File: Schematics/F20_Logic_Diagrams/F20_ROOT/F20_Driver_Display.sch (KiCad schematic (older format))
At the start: 2 parts, among them U5 StepDownConverter, U6 Driver_Display

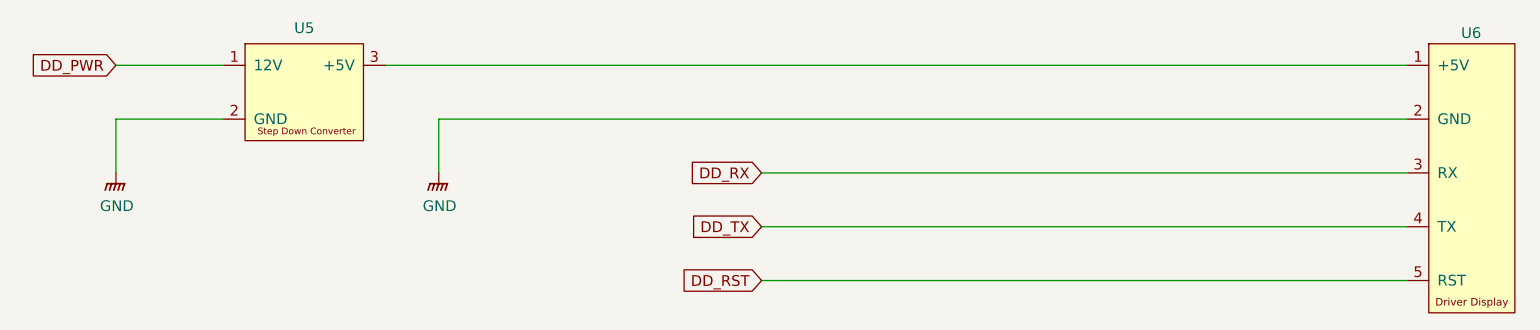
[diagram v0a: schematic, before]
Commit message: 02/18/20 update
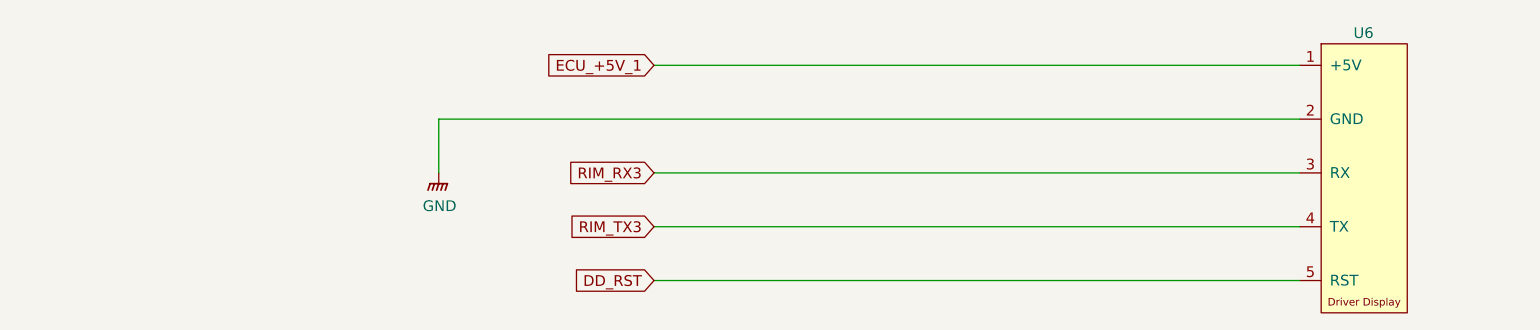
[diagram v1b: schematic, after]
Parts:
- removed U5: StepDownConverter, symbol FSAE_Library:StepDownConverter
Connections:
- net ECU_+5V_1: now reaches U6.1 (+5V)
- net DD_RX renamed RIM_RX3
- net DD_TX renamed RIM_TX3
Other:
- moved on the sheet: U6
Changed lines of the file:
@@
 $Descr A 11000 8500
 encoding utf-8
-Sheet 5 11
+Sheet 7 13
 Title "FSAE"
 Date "2020-02-03"
@@
 L FSAE_Library:Driver_Display U6
 U 1 1 5E291EA2
-P 8000 3000
-F 0 "U6" H 8250 3150 50  0000 L CNN
-F 1 "Driver_Display" H 8300 3150 50  0001 C CNN
-F 2 "" H 8300 3150 50  0001 C CNN
-F 3 "" H 8300 3150 50  0001 C CNN
-	1    8000 3000
-	1    0    0    -1
-$EndComp
-$Comp
-L FSAE_Library:StepDownConverter U5
-U 1 1 5E297DA5
-P 2500 3000
-F 0 "U5" H 2875 3173 50  0000 C CNN
-F 1 "StepDownConverter" H 2750 3150 50  0001 C CNN
-F 2 "" H 3000 3500 50  0001 C CNN
-F 3 "" H 3000 3500 50  0001 C CNN
-	1    2500 3000
+P 7500 3000
+F 0 "U6" H 7750 3150 50  0000 L CNN
+F 1 "Driver_Display" H 7800 3150 50  0001 C CNN
+F 2 "" H 7800 3150 50  0001 C CNN
+F 3 "" H 7800 3150 50  0001 C CNN
+	1    7500 3000
 	1    0    0    -1
 $EndComp
 Wire Wire Line
-	5000 3500 8000 3500
+	4500 3500 7500 3500
 Wire Wire Line
-	3250 3000 8000 3000
+	4500 3000 7500 3000
 Wire Wire Line
-	3500 3250 8000 3250
+	3500 3250 7500 3250
 Wire Wire Line
 	3500 3250 3500 3500
 Wire Wire Line
-	5000 3750 8000 3750
-Text GLabel 5000 4000 0    50   Input ~ 0
+	4500 3750 7500 3750
+Text GLabel 4500 4000 0    50   Input ~ 0
 DD_RST
 Wire Wire Line
-	5000 4000 8000 4000
-Wire Wire Line
-	2000 3500 2000 3250
-Wire Wire Line
-	2000 3250 2500 3250
-Text GLabel 2000 3000 0    50   Input ~ 0
-DD_PWR
-Wire Wire Line
-	2000 3000 2500 3000
+	4500 4000 7500 4000
 $Comp
-L FSAE_Library:GND #PWR0103
-U 1 1 5E3C0D7F
-P 2000 3500
-F 0 "#PWR0103" H 2000 3300 50  0001 C CNN
-F 1 "GND" H 2004 3346 50  0000 C CNN
-F 2 "" H 2000 3450 50  0001 C CNN
-F 3 "" H 2000 3450 50  0001 C CNN
-	1    2000 3500
-	1    0    0    -1
-$EndComp
-$Comp
-L FSAE_Library:GND #PWR0104
+L FSAE_Library:GND #PWR07
 U 1 1 5E3C11D7
 P 3500 3500
-F 0 "#PWR0104" H 3500 3300 50  0001 C CNN
+F 0 "#PWR07" H 3500 3300 50  0001 C CNN
 F 1 "GND" H 3504 3346 50  0000 C CNN
 F 2 "" H 3500 3450 50  0001 C CNN
@@
 	1    0    0    -1
 $EndComp
-Text GLabel 5000 3500 0    50   Input ~ 0
-DD_RX
-Text GLabel 5000 3750 0    50   Input ~ 0
-DD_TX
+Text GLabel 4500 3500 0    50   Input ~ 0
+RIM_RX3
+Text GLabel 4500 3750 0    50   Input ~ 0
+RIM_TX3
+Text GLabel 4500 3000 0    50   Input ~ 0
+ECU_+5V_1
 $EndSCHEMATC

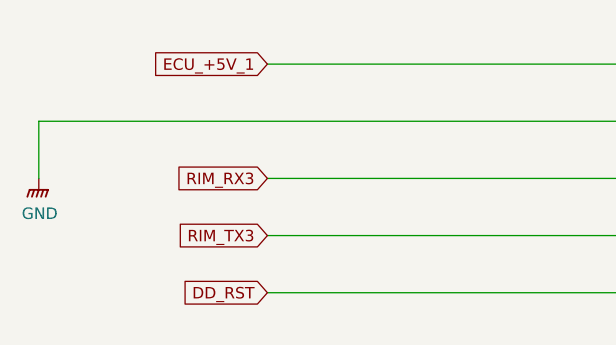
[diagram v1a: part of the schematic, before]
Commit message: 02/19/20 update
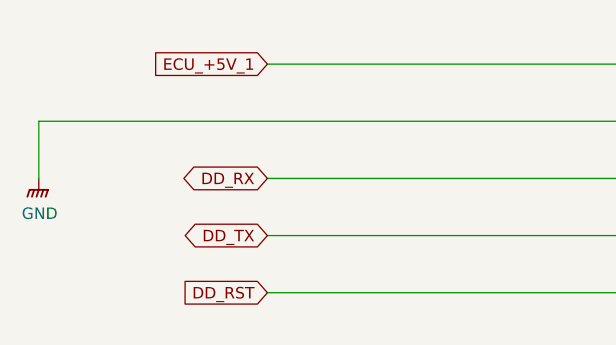
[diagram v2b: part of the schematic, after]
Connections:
- net RIM_RX3 renamed DD_RX
- net RIM_TX3 renamed DD_TX
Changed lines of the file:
@@
 	1    0    0    -1
 $EndComp
-Text GLabel 4500 3500 0    50   Input ~ 0
-RIM_RX3
-Text GLabel 4500 3750 0    50   Input ~ 0
-RIM_TX3
+Text GLabel 4500 3500 0    50   BiDi ~ 0
+DD_RX
 Text GLabel 4500 3000 0    50   Input ~ 0
 ECU_+5V_1
+Text GLabel 4500 3750 0    50   BiDi ~ 0
+DD_TX
 $EndSCHEMATC
